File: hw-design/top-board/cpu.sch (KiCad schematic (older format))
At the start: 24 parts

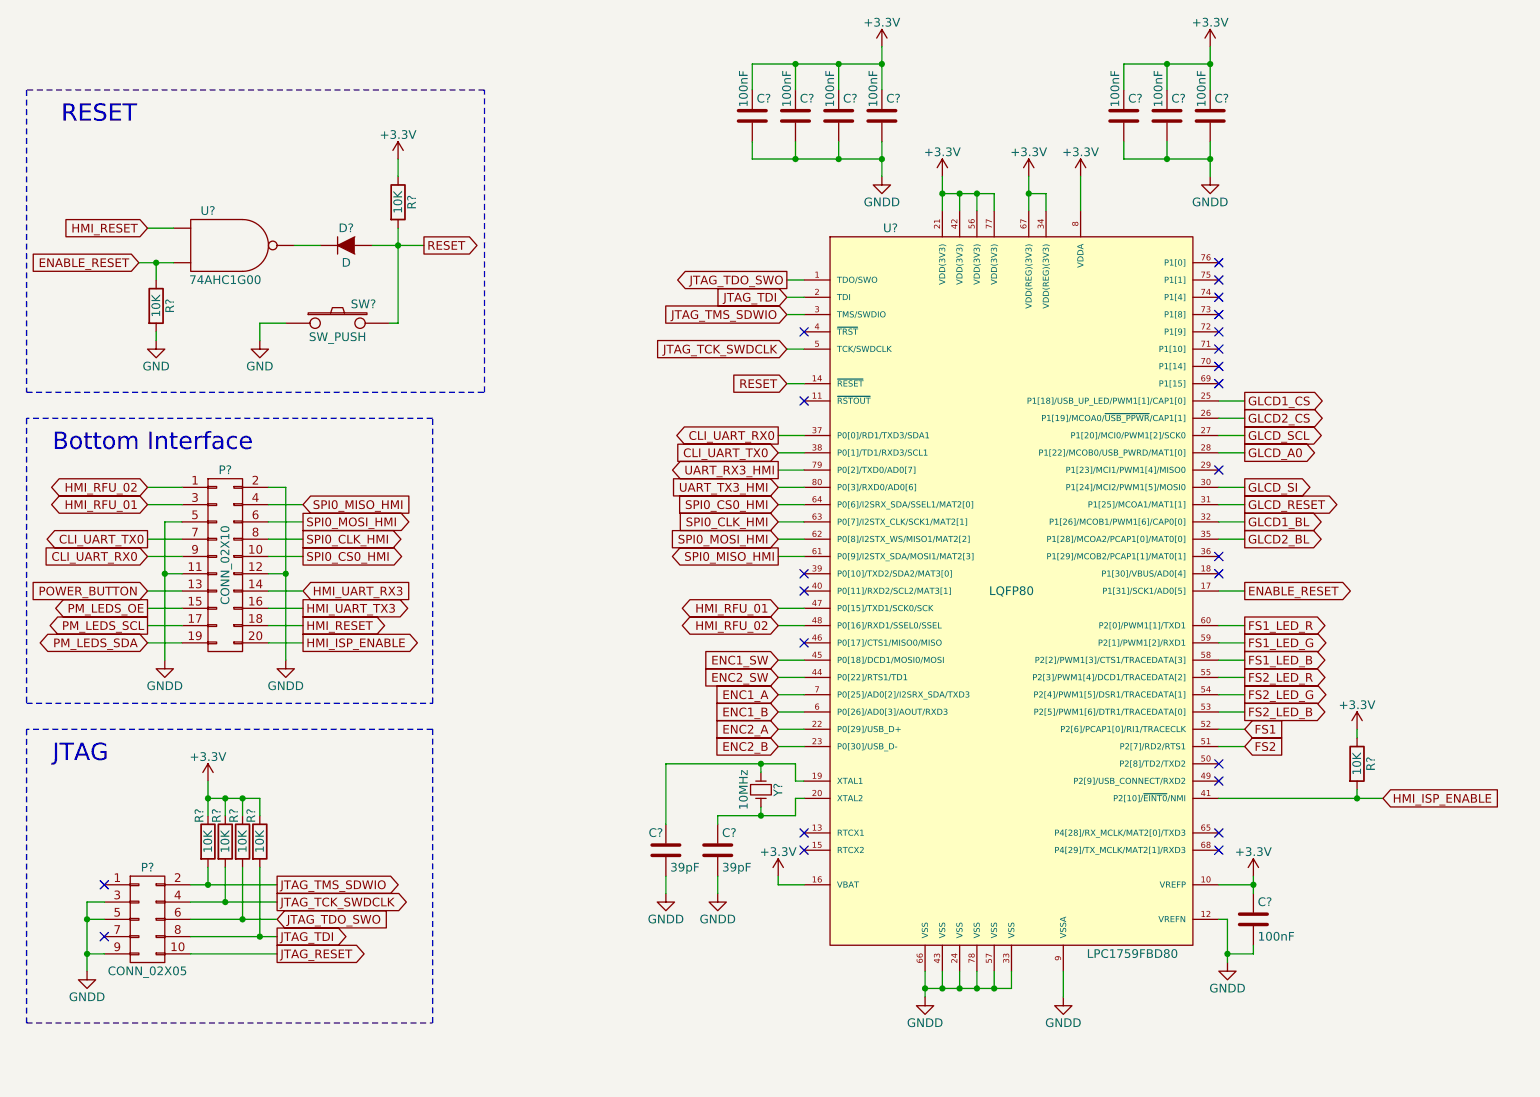
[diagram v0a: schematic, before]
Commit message: sch,top-board: annotation done
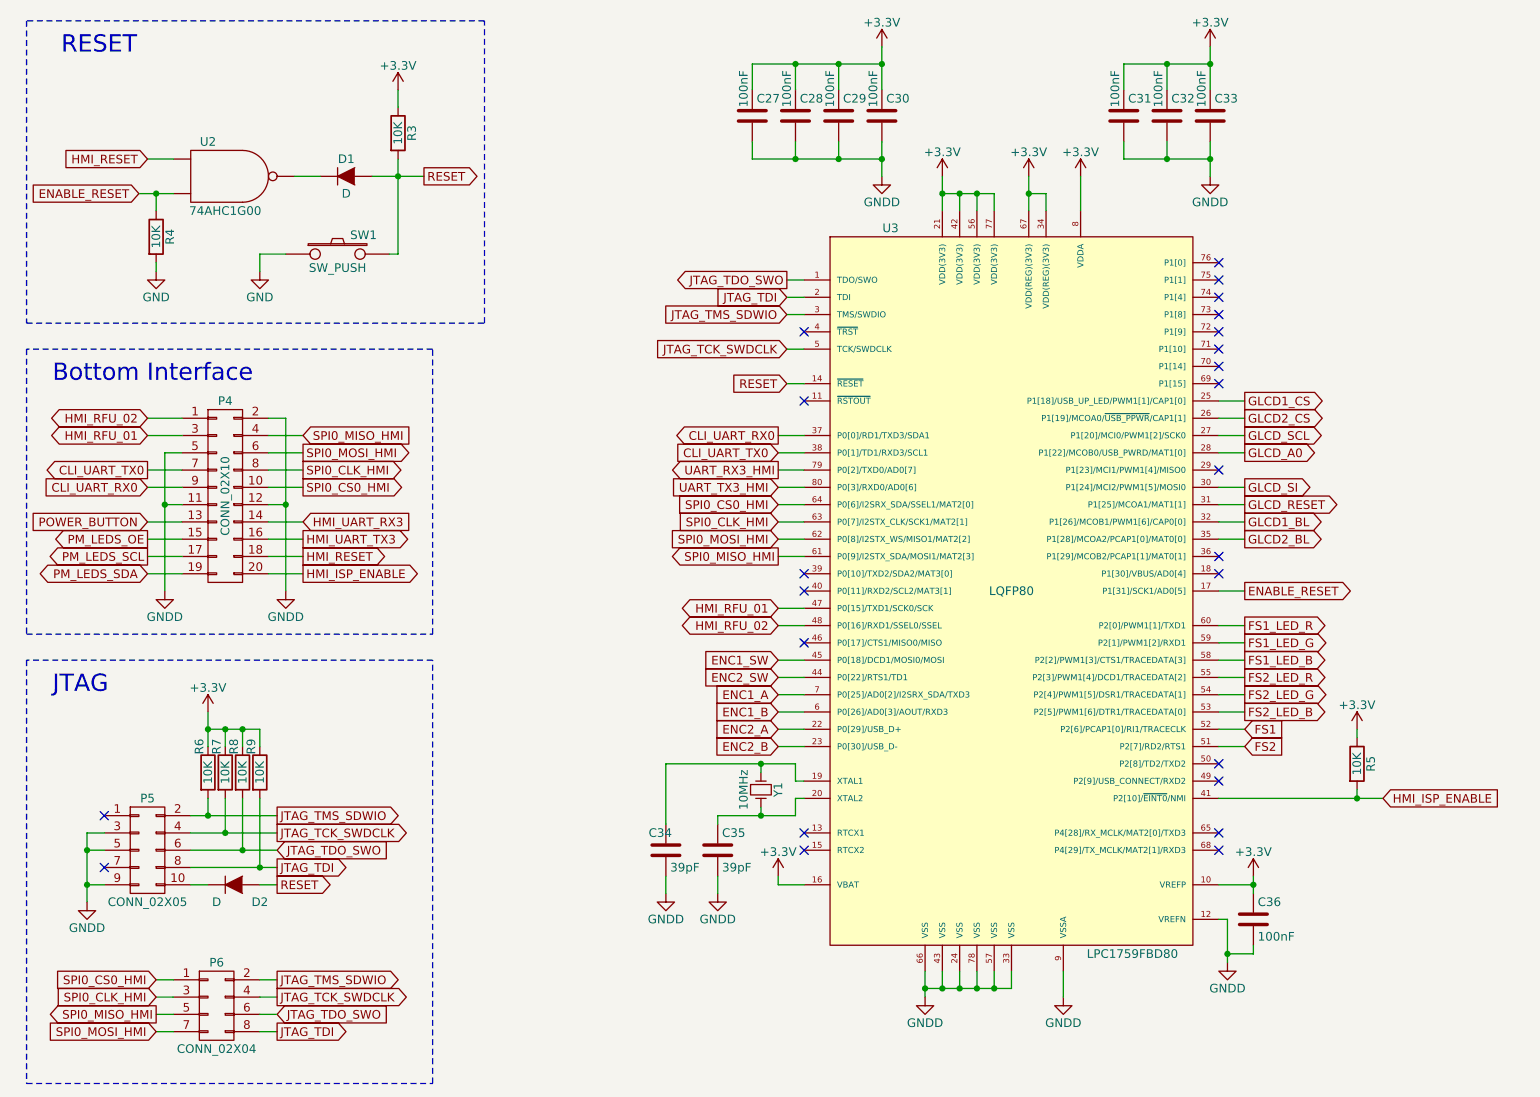
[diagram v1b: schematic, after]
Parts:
- added D2: D, symbol D
- added P6: CONN_02X04, symbol CONN_02X04
- gave numbers to parts that had none: 24
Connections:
- net JTAG_TCK_SWDCLK: now also P6.4 (P4)
- net JTAG_TDI: now also P6.8 (P8)
- net JTAG_TDO_SWO: now also P6.6 (P6)
- net JTAG_TMS_SDWIO: now also P6.2 (P2)
- net RESET: now also D2.2 (A)
- net SPI0_CLK_HMI: now also P6.3 (P3)
- net SPI0_CS0_HMI: now also P6.1 (P1)
- net SPI0_MISO_HMI: now also P6.5 (P5)
- net SPI0_MOSI_HMI: now also P6.7 (P7)
- net JTAG_RESET: no longer names the net of P5.10 (P10)
- net JTAG_RESET: now also D2.1 (K)
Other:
- moved on the sheet: D1, P4, P5, R3, R4, R6, R7, R8, R9, SW1, U2
